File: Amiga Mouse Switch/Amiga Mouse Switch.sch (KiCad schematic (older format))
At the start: 24 parts, among them J1 JOYSTICK, J2 Mouse, J3 Amiga IDC, M1 Mounting, M2 Mounting, M3 Mounting, M4 Mounting, SW1 JOY_SEL, SW2 MOUSE_SEL, U1 74HCT4053, U2 74HCT4053, U3 NE555

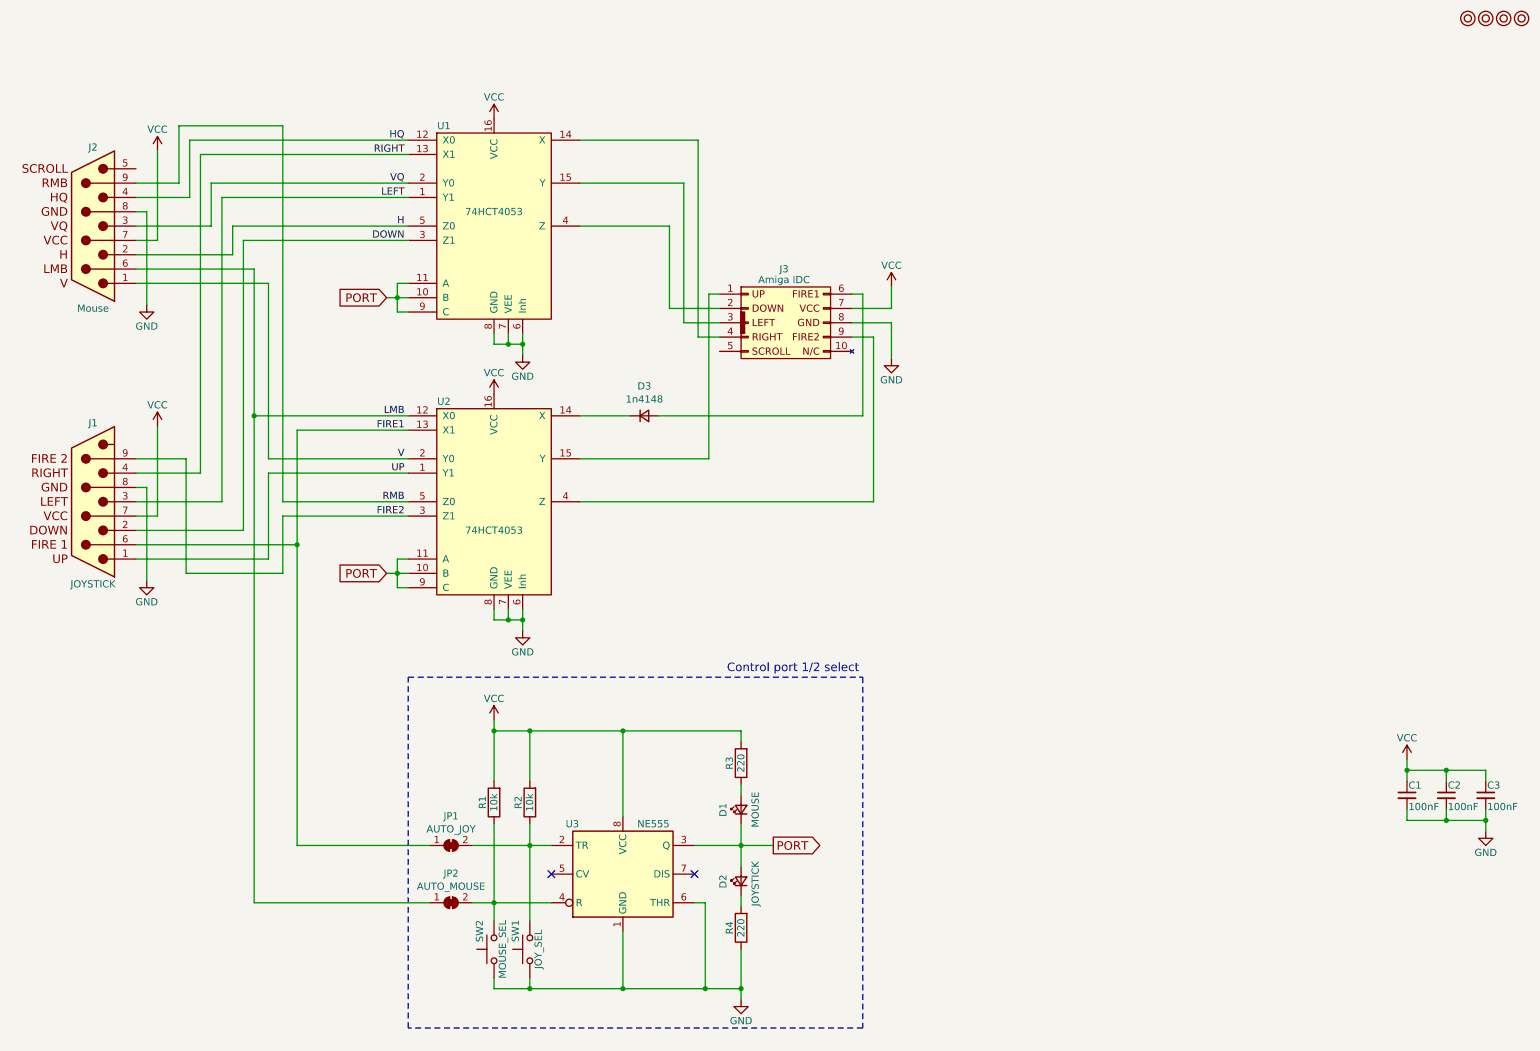
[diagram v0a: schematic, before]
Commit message: Fixed RMB
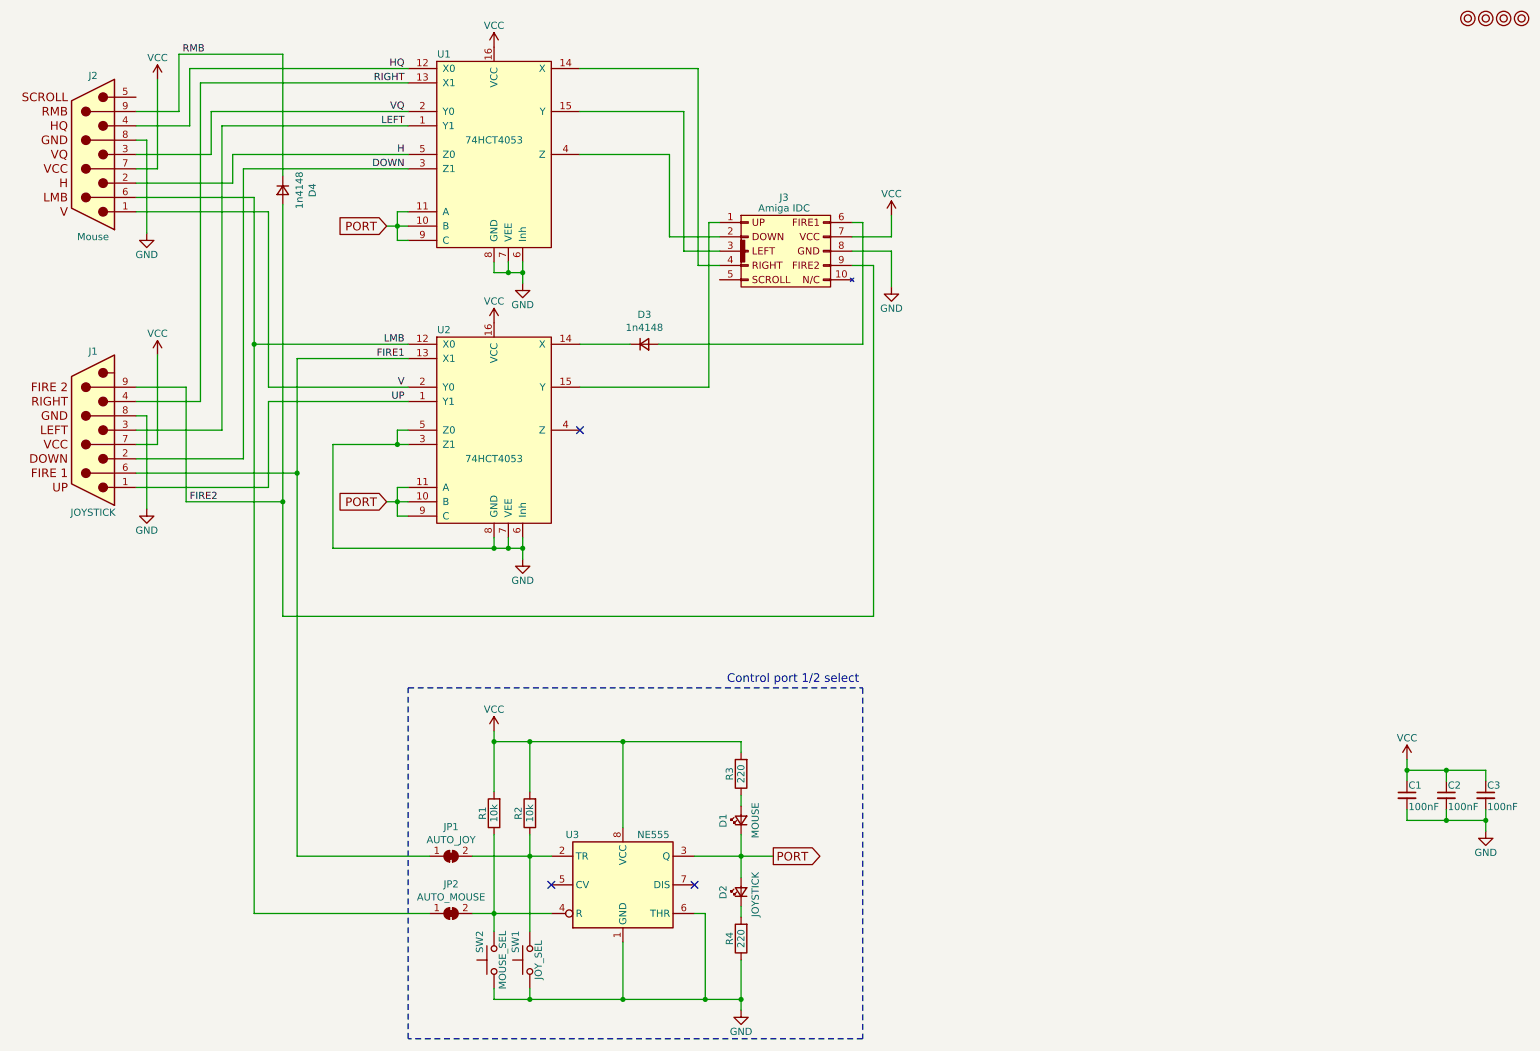
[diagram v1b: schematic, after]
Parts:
- added D4: 1n4148, Diode_THT:D_DO-35_SOD27_P7.62mm_Horizontal, symbol Device:D_Small
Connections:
- net FIRE2: now also J3.9 (Pin_9), D4.2 (A); no longer U2.3 (Z1)
- net GND: now also U2.3 (Z1), U2.5 (Z0)
- net RMB: now also D4.1 (K); no longer U2.5 (Z0)
- net at U2.4 (Z): no longer J3.9 (Pin_9)
- no-connect marks 2 -> 3
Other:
- moved on the sheet: D1, D2, D3, J1, J2, J3, JP1, JP2, R1, R2, R3, R4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
